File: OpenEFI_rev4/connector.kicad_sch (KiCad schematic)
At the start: 30 parts, among them J6 1241434-1, Q10 IRF540N, Q19 PMOS, Q5 SS8050, Q6 IRLZ44N, Q7 IRLZ44N, U14 MIC5205-3.3YM5, U4 MIC2940A-3.3WU, U5 MIC2940A-5.0WT, U6 LT4363IMS

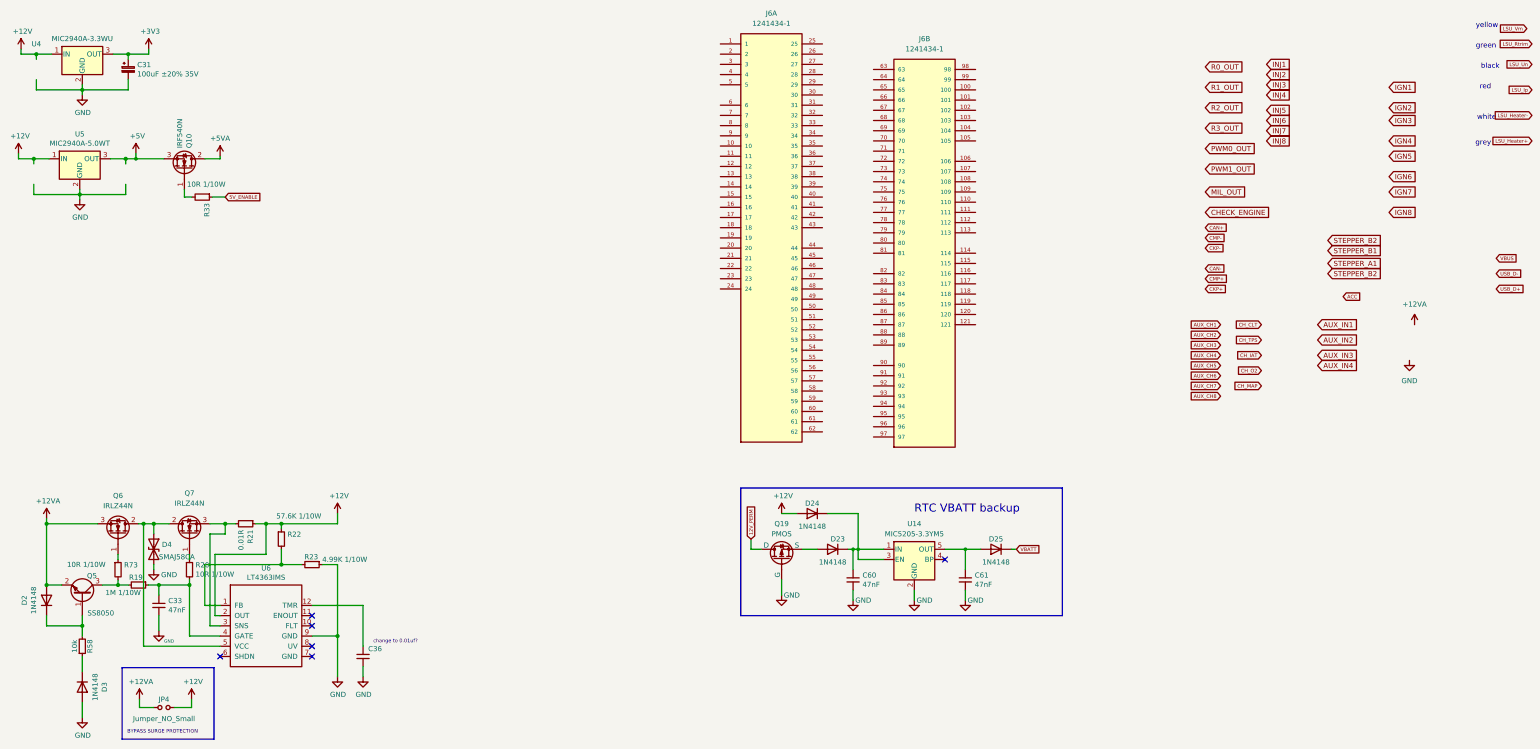
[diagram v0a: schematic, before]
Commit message: WIP Analog frontend
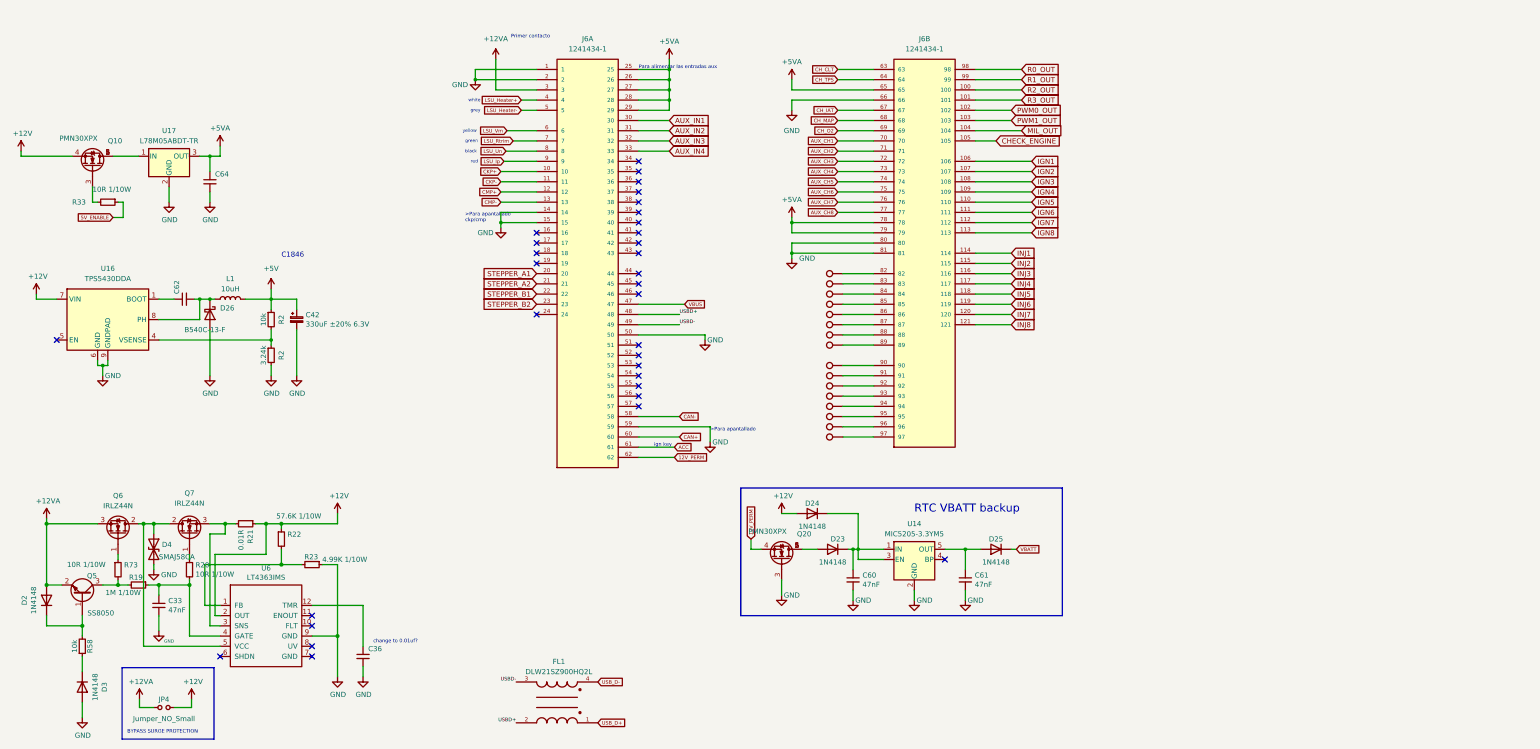
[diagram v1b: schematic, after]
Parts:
- removed C31: 100uF ±20% 35V, Capacitor_SMD:CP_Elec_6.3x7.7, symbol Device:CP_Small
- removed Q19: PMOS, Package_TO_SOT_SMD:SOT-23-3, symbol Simulation_SPICE:PMOS
- removed U4: MIC2940A-3.3WU, Package_TO_SOT_SMD:TO-263-3_TabPin2, symbol Regulator_Linear:L7805
- removed U5: MIC2940A-5.0WT, Package_TO_SOT_THT:TO-220-3_Vertical, symbol Regulator_Linear:L7805
- added C42: 330uF ±20% 6.3V, Capacitor_SMD:CP_Elec_6.3x7.7, symbol Device:CP_Small
- added C62: 10nF, Capacitor_SMD:C_0805_2012Metric, symbol Device:C_Small
- added C64: 100nF, Capacitor_SMD:C_0805_2012Metric, symbol Device:C_Small
- added D26: B540C-13-F, Diode_SMD:D_SMA, symbol Device:D_Schottky
- added FL1: DLW21SZ900HQ2L, Library:FIL_DLW21SZ900HQ2L, symbol Library:DLW21SZ900HQ2L
- added L1: 10uH, Inductor_SMD:L_7.3x7.3_H4.5, symbol Device:L
- added Q20: PMN30XPX, Package_SO:TSOP-6_1.65x3.05mm_P0.95mm, symbol Transistor_FET:IRF540N
- added R2: 10k, Resistor_SMD:R_0603_1608Metric, symbol Device:R_Small
- added R2: 3.24k, Resistor_SMD:R_0603_1608Metric, symbol Device:R_Small
- added TP22, TP24, TP26, TP27, TP31, TP32, TP33, TP34, TP67, TP68, TP69, TP70, TP71, TP72, TP73, TP74: TestPoint, TestPoint:TestPoint_THTPad_1.5x1.5mm_Drill0.7mm, symbol Connector:TestPoint
- added U16: TPS5430DDA, Package_SO:TI_SO-PowerPAD-8_ThermalVias, symbol Regulator_Switching:TPS5430DDA
- added U17: L78M05ABDT-TR, Package_TO_SOT_SMD:TO-252-2, symbol Regulator_Linear:L7805
- Q10: value IRF540N -> PMN30XPX; footprint Package_TO_SOT_THT:TO-220-3_Vertical -> Package_SO:TSOP-6_1.65x3.05mm_P0.95mm; LCSC (none) -> C5288813
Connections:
- net +12V: now also Q10.4 (S), U16.7 (VIN)
- net +12VA: now also J6.3
- net +5V: now also C42.1, L1.2, R2.1; no longer Q10.3 (S)
- net +5VA: now also J6.25, J6.26, J6.27, J6.28, J6.29, J6.65, J6.78, J6.79, C64.1, U17.3 (OUT); no longer Q10.2 (D)
- net 12V_PERM: now also J6.62, Q20.4 (S)
- net ACC: now also J6.61
- net AUX_CH1: now also J6.70
- net AUX_CH2: now also J6.71
- net AUX_CH3: now also J6.72
- net AUX_CH4: now also J6.73
- net AUX_CH5: now also J6.74
- net AUX_CH6: now also J6.75
- net AUX_CH7: now also J6.76
- net AUX_CH8: now also J6.77
- net AUX_IN1: now also J6.30
- net AUX_IN2: now also J6.31
- net AUX_IN3: now also J6.32
- net AUX_IN4: now also J6.33
- net CAN+: now also J6.60
- net CAN-: now also J6.58
- net CHECK_ENGINE: now also J6.105
- net CH_CLT: now also J6.63
- net CH_IAT: now also J6.67
- net CH_MAP: now also J6.68
- net CH_O2: now also J6.69
- net CH_TPS: now also J6.64
- net CKP+: now also J6.10
- net CKP-: now also J6.11
- net CMP+: now also J6.12
- net CMP-: now also J6.13
- net GND: now also J6.1, J6.14, J6.15, J6.2, J6.50, J6.59, J6.66, J6.80, J6.81, C42.2, C64.2, D26.2 (A), Q20.3 (G), R2.2, U16.6 (GND), U16.9 (GNDPAD), U17.2 (GND)
- net IGN1: now also J6.106
- net IGN2: now also J6.107
- net IGN3: now also J6.108
- net IGN4: now also J6.109
- net IGN5: now also J6.110
- net IGN6: now also J6.111
- net IGN7: now also J6.112
- net IGN8: now also J6.113
- net INJ1: now also J6.114
- net INJ2: now also J6.115
- net INJ3: now also J6.116
- net INJ4: now also J6.117
- net INJ5: now also J6.118
- net INJ6: now also J6.119
- net INJ7: now also J6.120
- net INJ8: now also J6.121
- net LSU_Heater+: now also J6.4
- net LSU_Heater-: now also J6.5
- net LSU_Ip: now also J6.9
- net LSU_Rtrim: now also J6.7
- net LSU_Un: now also J6.8
- net LSU_Vm: now also J6.6
- net MIL_OUT: now also J6.104
- net PWM0_OUT: now also J6.102
- net PWM1_OUT: now also J6.103
- net R0_OUT: now also J6.98
- net R1_OUT: now also J6.99
- net R2_OUT: now also J6.100
- net R3_OUT: now also J6.101
- net STEPPER_A1: now also J6.20
- net STEPPER_B1: now also J6.22
- net STEPPER_B2: now also J6.23
- net USB_D+: now also FL1.1
- net USB_D-: now also FL1.4
- net VBUS: now also J6.47
- net at R33.2: now also Q10.3 (G); no longer Q10.1 (G)
- net at J6.82: now also TP34.1
- net at J6.83: now also TP33.1
- net at J6.84: now also TP32.1
- net at J6.85: now also TP31.1
- net at J6.86: now also TP27.1
- net at J6.87: now also TP26.1
- net at J6.88: now also TP24.1
- net at J6.89: now also TP22.1
- net at J6.90: now also TP74.1
- net at J6.91: now also TP73.1
- net at J6.92: now also TP72.1
- net at J6.93: now also TP71.1
- net at J6.94: now also TP70.1
- net at J6.95: now also TP69.1
- net at J6.96: now also TP68.1
- net at J6.97: now also TP67.1
- net at D23.2 (A): now also Q20.1 (D), Q20.2 (D), Q20.5 (D), Q20.6 (D)
- net STEPPER_A2: now reaches J6.21
- net USBD+: now reaches J6.48
- net USBD+: now also FL1.2
- net USBD-: now reaches J6.49
- net USBD-: now also FL1.3
- new net: C62.2, D26.1 (K), L1.1, U16.8 (PH)
- new net: C62.1, U16.1 (BOOT)
- new net: R2.1, R2.2, U16.4 (VSENSE)
- new net: Q10.1 (D), Q10.2 (D), Q10.5 (D), Q10.6 (D), U17.1 (IN)
- no-connect marks 6 -> 32
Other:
- note added: ">Para apantallado"
- note added: ">Para apantallado ckp/cmp"
- note added: "C1846"
- note added: "Para alimentar las entradas aux"
- note added: "Primer contacto"
- note added: "ign key"
- moved on the sheet: J6A, R33
